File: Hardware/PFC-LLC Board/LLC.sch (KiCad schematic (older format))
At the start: 83 parts, among them J4 1792229, J5 Conn_01x02_Female, J6 1792229, U1LLC1 UCC256403DDBR, U2LLC1 UCC24624DT

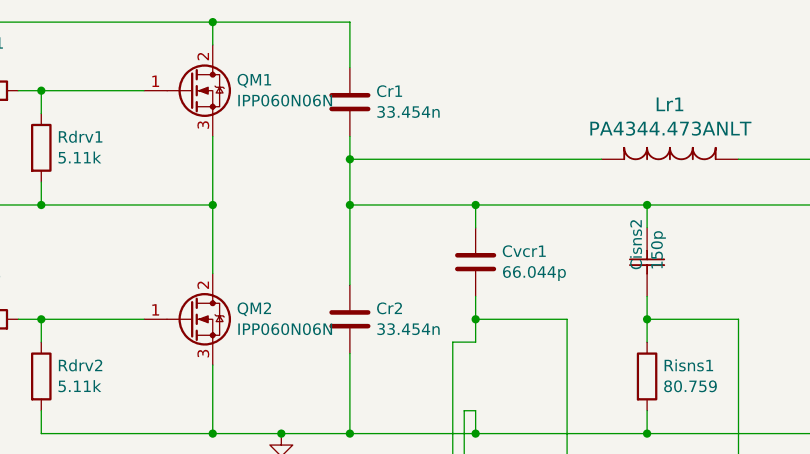
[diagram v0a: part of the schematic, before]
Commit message: Gerber files generated
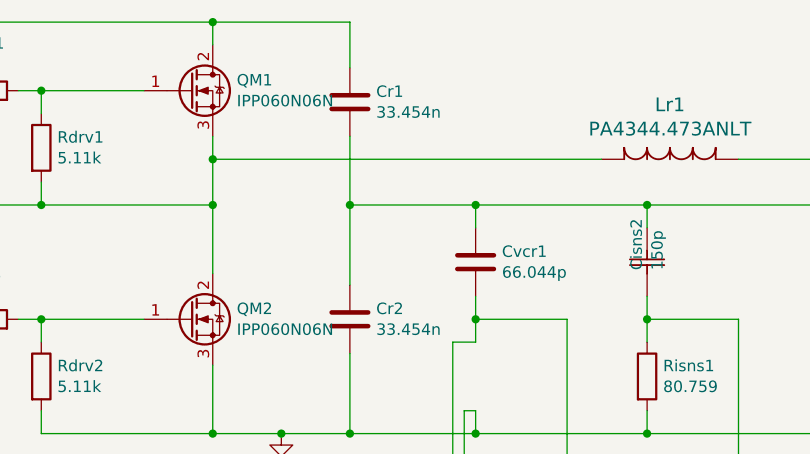
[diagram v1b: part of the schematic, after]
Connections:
- net HS: now also Lr1.2
- net at Cisns2.2, Cr1.2, Cr2.1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: no longer Lr1.2
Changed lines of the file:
@@
 	6850 1850 8200 1850
-Wire Wire Line
-	5150 1750 5150 1850
 Wire Wire Line
 	8200 2050 6450 2050
@@
 $EndComp
 Wire Wire Line
-	4550 1750 4550 2050
-Wire Wire Line
-	6250 1850 5150 1850
-Connection ~ 5150 1850
-Wire Wire Line
-	5150 1850 5150 2050
+	4550 1750 4550 1850
 $Comp
 L Connector2x1:1792229 J?
@@
 Wire Wire Line
 	7350 5700 6850 5700
+Wire Wire Line
+	5150 1750 5150 2050
+Wire Wire Line
+	6250 1850 4550 1850
+Connection ~ 4550 1850
+Wire Wire Line
+	4550 1850 4550 2050
 $EndSCHEMATC
